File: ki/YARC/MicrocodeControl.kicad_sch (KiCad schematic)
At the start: 11 parts, among them U54 74LS32, U56 74LS574, U57 74LS157, U58 74LS157, U59 74LS193, U60 74LS193, U61 74LS139, U62 74LS32, U63 74LS32, U64 74LS157, U65 74LS32

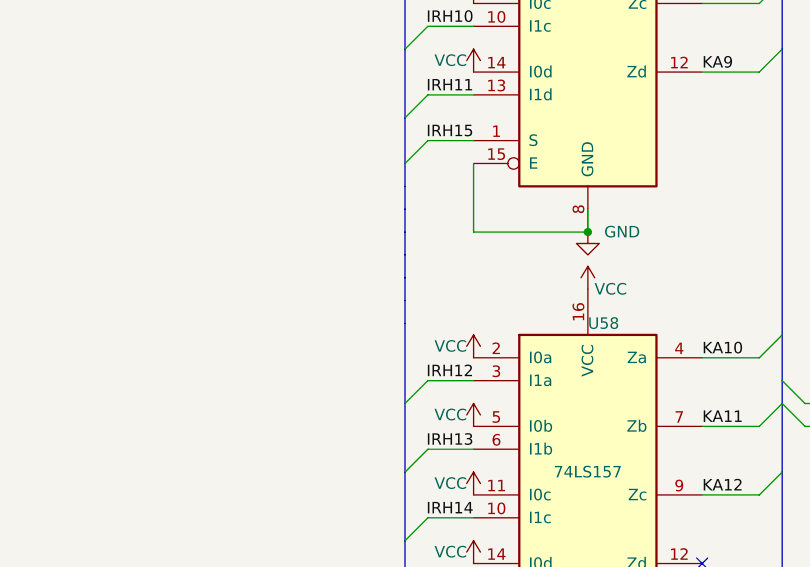
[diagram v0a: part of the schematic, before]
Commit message: Continuing cleanup of schematic
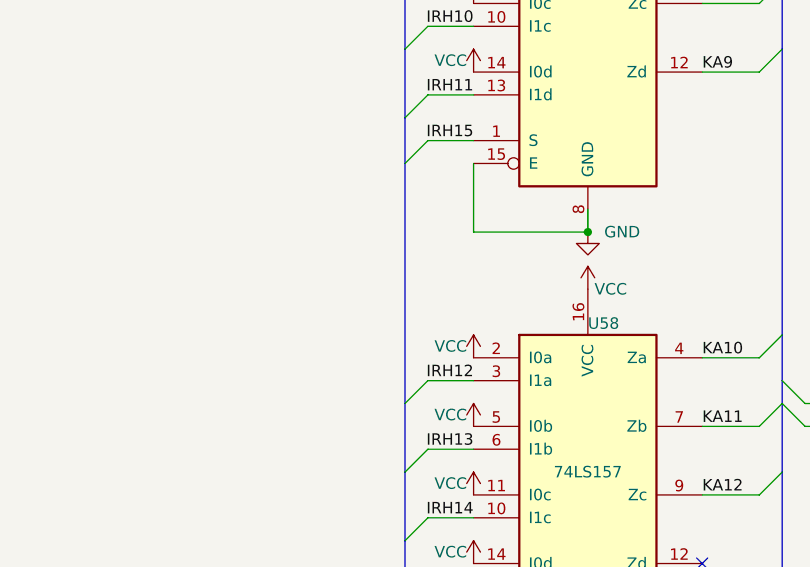
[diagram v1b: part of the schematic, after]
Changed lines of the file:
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@@
     (stroke (width 0) (type default))
   )
-  (bus (pts (xy 60.96 152.4) (xy 60.96 161.29))
+  (bus (pts (xy 60.96 134.62) (xy 60.96 161.29))
     (stroke (width 0) (type default))
   )
@@
     (stroke (width 0) (type default))
   )
-  (bus (pts (xy 60.96 144.78) (xy 60.96 147.32))
-    (stroke (width 0) (type default))
-  )
   (wire (pts (xy 137.16 166.37) (xy 137.16 163.83))
     (stroke (width 0) (type default))
@@
     (stroke (width 0) (type default))
   )
-  (bus (pts (xy 60.96 142.24) (xy 60.96 144.78))
-    (stroke (width 0) (type default))
-  )
   (wire (pts (xy 137.16 105.41) (xy 137.16 107.95))
     (stroke (width 0) (type default))
@@
     (stroke (width 0) (type default))
   )
-  (bus (pts (xy 60.96 139.7) (xy 60.96 142.24))
-    (stroke (width 0) (type default))
-  )
   (wire (pts (xy 105.41 161.29) (xy 111.76 161.29))
     (stroke (width 0) (type default))
@@
     (stroke (width 0) (type default))
   )
-  (bus (pts (xy 60.96 134.62) (xy 60.96 137.16))
-    (stroke (width 0) (type default))
-  )
   (wire (pts (xy 228.6 24.13) (xy 245.11 24.13))
     (stroke (width 0) (type default))
@@
     (stroke (width 0) (type default))
   )
-  (bus (pts (xy 60.96 147.32) (xy 60.96 149.86))
-    (stroke (width 0) (type default))
-  )
   (wire (pts (xy 166.37 57.15) (xy 173.99 57.15))
     (stroke (width 0) (type default))
@@
     (stroke (width 0) (type default))
   )
-  (bus (pts (xy 60.96 149.86) (xy 60.96 152.4))
-    (stroke (width 0) (type default))
-  )
   (wire (pts (xy 55.88 45.72) (xy 111.76 45.72))
     (stroke (width 0) (type default))
@@
     (stroke (width 0) (type default))
   )
-  (bus (pts (xy 60.96 137.16) (xy 60.96 139.7))
-    (stroke (width 0) (type default))
-  )
